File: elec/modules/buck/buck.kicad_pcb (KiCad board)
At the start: 2 copper layers, 40.6 x 30.5 mm, 11 parts, among them J1 Conn_01x12

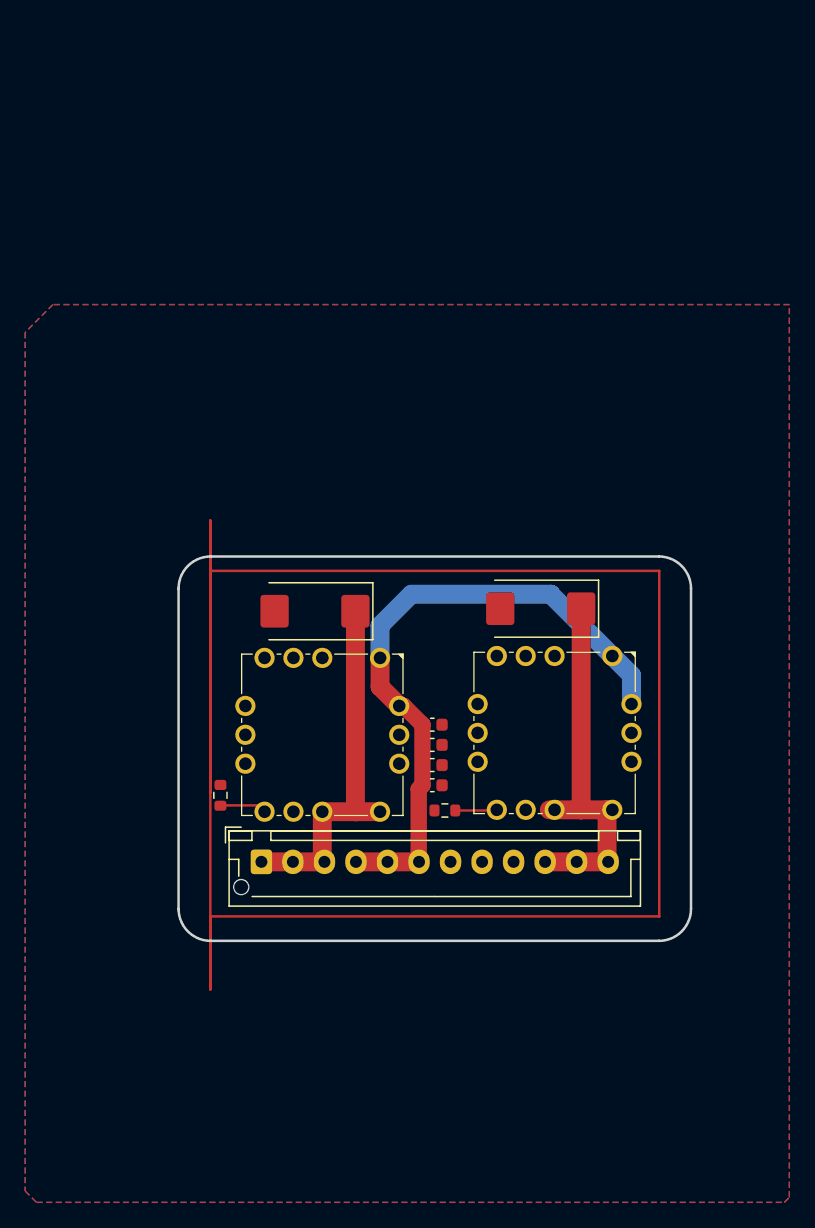
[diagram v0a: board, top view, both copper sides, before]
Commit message: Revert "buck seems done idk"
This reverts commit 98c0c33bcc0f6ab69bf7f0e82d9e932e885d420a.
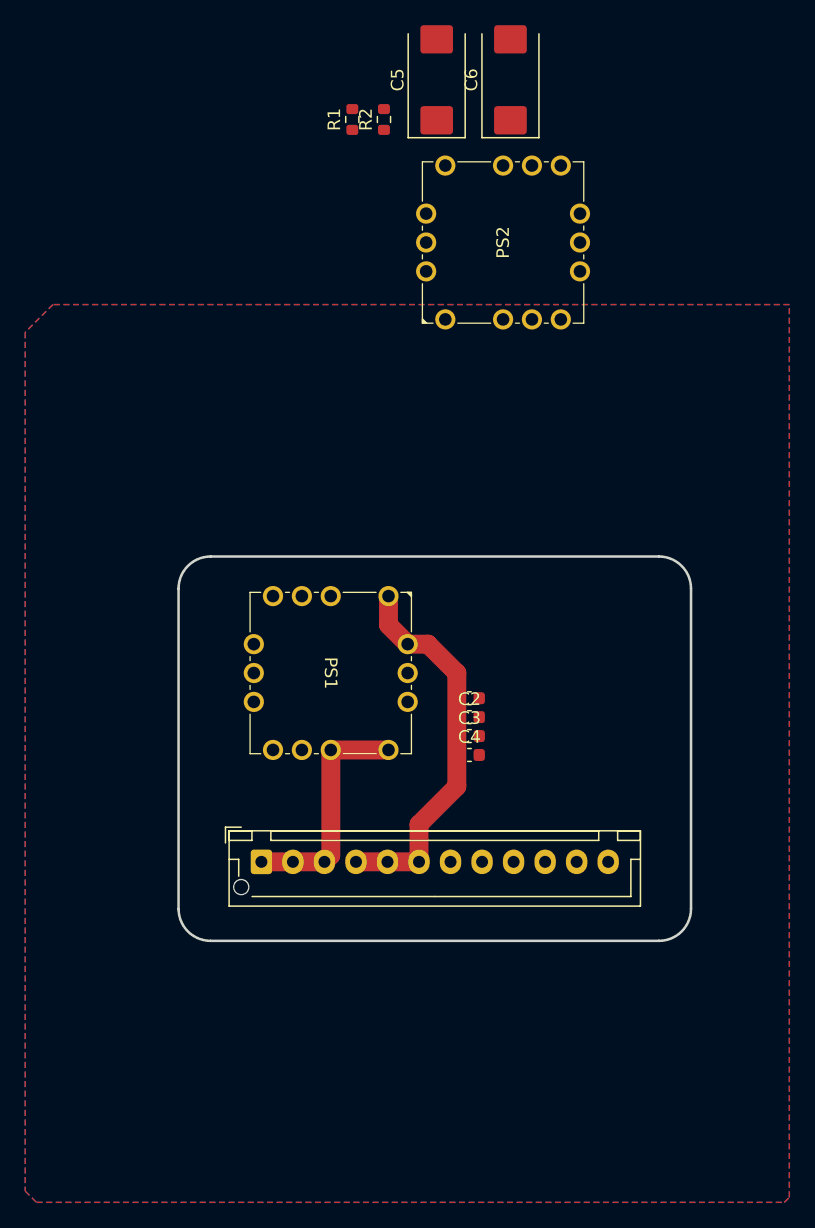
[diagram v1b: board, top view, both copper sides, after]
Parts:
- moved R2 55.0 mm to (145.2, 50.4), turned to 90 degrees
- moved R1 54.6 mm to (142.7, 50.4)
- moved C5 43.2 mm to (149.4, 47.2), turned to 90 degrees
- moved C6 42.0 mm to (155.3, 47.2), turned to 90 degrees
- moved PS2 39.1 mm to (154.7, 60.1), turned to 90 degrees
- moved PS1 4.95 mm to (141.0, 94.3)
- moved C4 3.80 mm to (152.0, 100.8)
- moved C3 3.74 mm to (152.0, 99.3)
- moved C2 3.68 mm to (152.0, 97.8)
- moved C1 3.62 mm to (152.0, 96.3)
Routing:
- net +3V3: track 29.7 -> 0.00 mm
- net +12V: track 51.4 -> 30.5 mm
- net +5V: track 29.9 -> 18.7 mm
- net Net-(PS1-TRIM): track 3.34 -> 0.00 mm
- net Net-(PS2-TRIM): track 3.32 -> 0.00 mm

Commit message: buck seems done idk
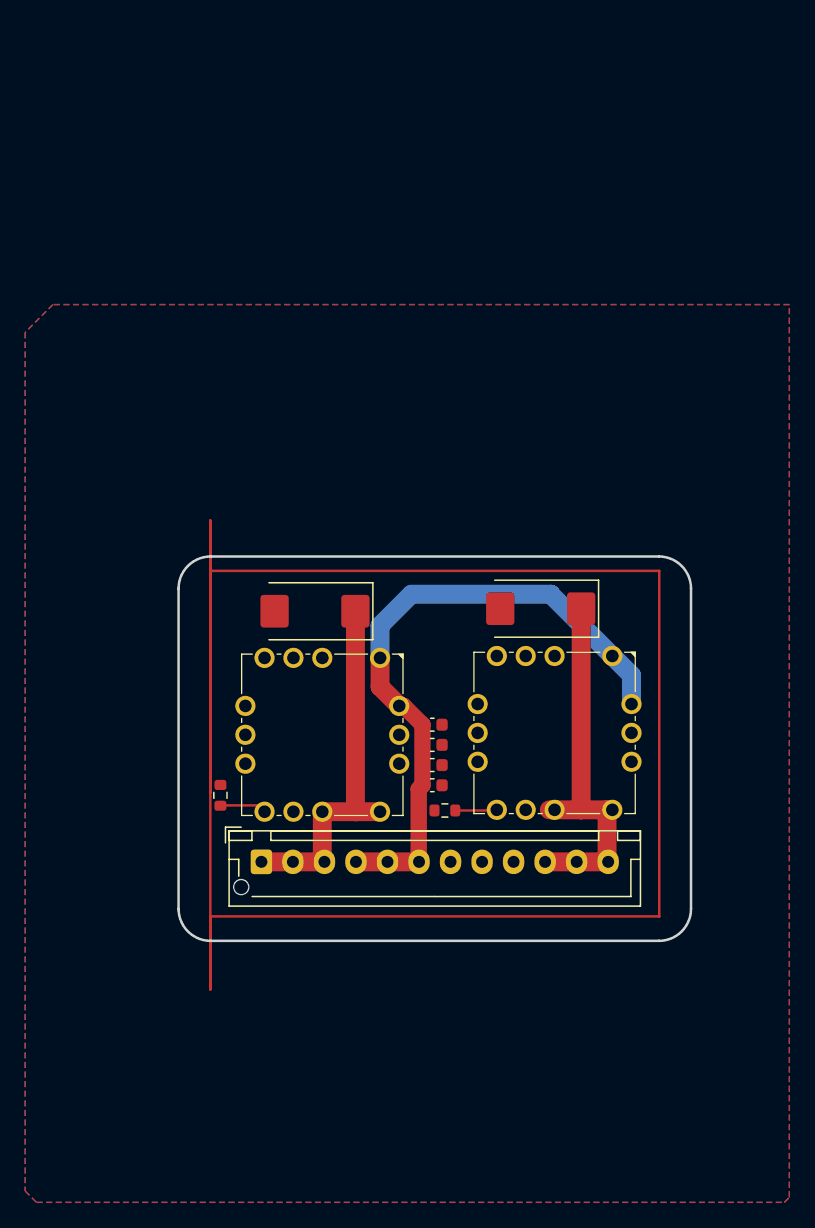
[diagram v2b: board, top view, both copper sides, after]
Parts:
- moved R2 55.0 mm to (150.1, 105.2), turned to 180 degrees
- moved R1 54.6 mm to (132.3, 104.0)
- moved C5 43.2 mm to (139.8, 89.4), turned to 180 degrees
- moved C6 42.0 mm to (157.7, 89.2), turned to 180 degrees
- moved PS2 39.1 mm to (158.8, 99.0), turned to -90 degrees
- moved PS1 4.95 mm to (140.4, 99.2)
- moved C4 3.80 mm to (149.1, 103.2)
- moved C3 3.74 mm to (149.1, 101.6)
- moved C2 3.68 mm to (149.1, 100.0)
- moved C1 3.62 mm to (149.1, 98.4)
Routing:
- net +3V3: track 0.00 -> 29.7 mm
- net +12V: track 30.5 -> 51.4 mm
- net +5V: track 18.7 -> 29.9 mm
- net Net-(PS1-TRIM): track 0.00 -> 3.34 mm
- net Net-(PS2-TRIM): track 0.00 -> 3.32 mm
